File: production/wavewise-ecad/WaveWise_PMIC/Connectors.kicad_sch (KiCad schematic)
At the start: 30 parts, among them J1 5031590200, J10 5031590200, J11 5031590200, J13 Screw_Terminal_01x03, J2 Conn_01x06_Pin, J3 Conn_01x03_Pin, J5 5031590400, J6 5031590400, J8 5031590800, J9 5031590300

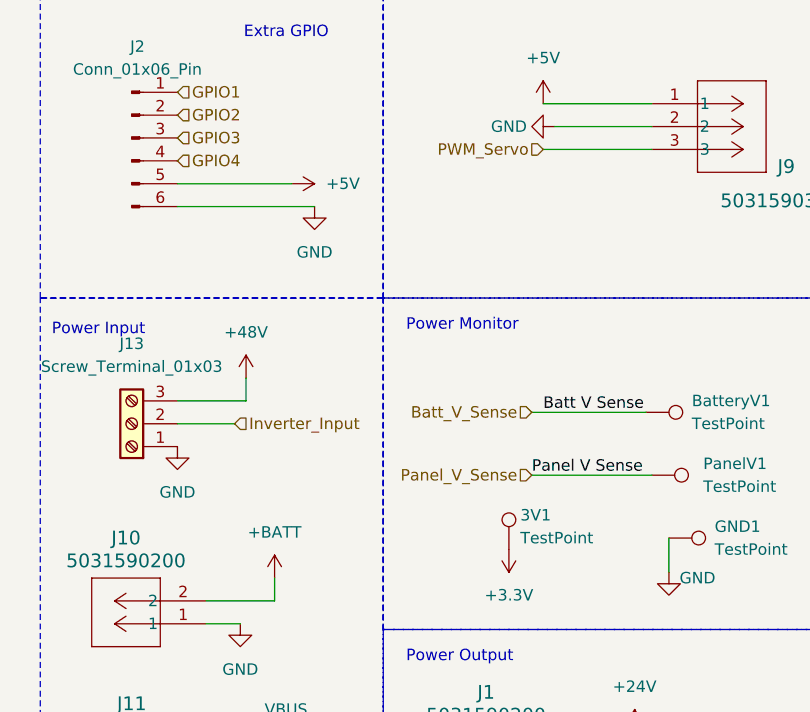
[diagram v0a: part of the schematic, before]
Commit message: add gerber files
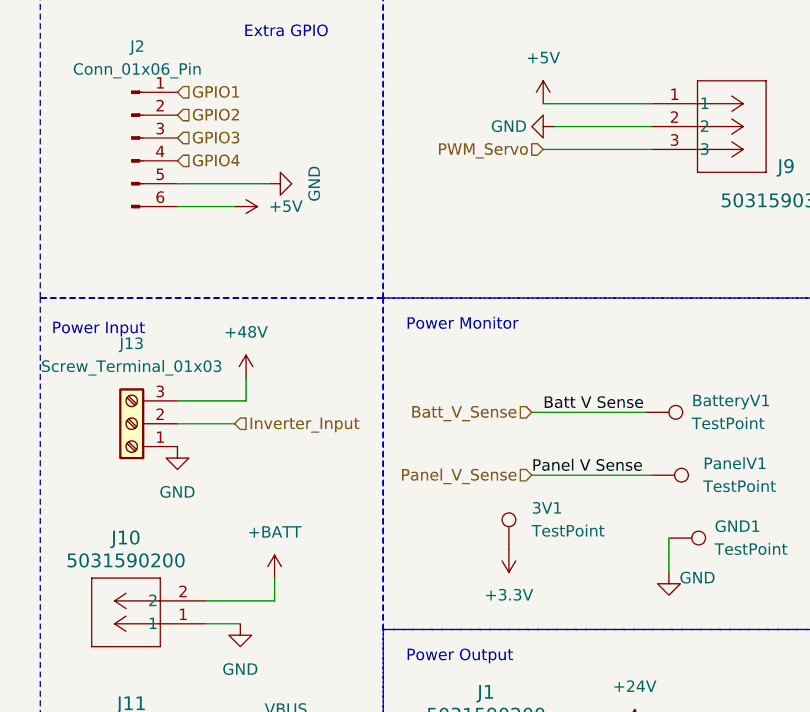
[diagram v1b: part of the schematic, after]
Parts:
- 3V1: footprint TestPoint:TestPoint_Pad_D1.5mm -> TestPoint:TestPoint_THTPad_D2.0mm_Drill1.0mm
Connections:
- net +5V: now also J2.6 (Pin_6); no longer J2.5 (Pin_5)
- net GND: now also J2.5 (Pin_5); no longer J2.6 (Pin_6)
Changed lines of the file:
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@@
   (junction (at 157.48 106.68) (diameter 0) (color 0 0 0 0)
+  )
+  (wire (pts (xy 27.94 39.37) (xy 34.29 39.37))
+    (stroke (width 0) (type default))
   )
   (polyline (pts (xy 105.41 123.19) (xy 105.41 126.746))
@@
     (stroke (width 0) (type default))
   )
+  (wire (pts (xy 27.94 36.83) (xy 38.1 36.83))
+    (stroke (width 0) (type default))
+  )
   (wire (pts (xy 78.74 138.43) (xy 78.74 139.7))
     (stroke (width 0) (type default))
@@
     (stroke (width 0) (type default))
   )
-  (wire (pts (xy 43.18 39.37) (xy 27.94 39.37))
-    (stroke (width 0) (type default))
-  )
   (wire (pts (xy 158.75 114.3) (xy 157.48 114.3))
     (stroke (width 0) (type default))
@@
   )
   (wire (pts (xy 120.904 84.328) (xy 128.016 84.328))
-    (stroke (width 0) (type default))
-  )
-  (wire (pts (xy 40.64 36.83) (xy 27.94 36.83))
     (stroke (width 0) (type default))
   )
@@
     )
   )
+  (symbol (lib_id "Connector:TestPoint") (at 64.77 77.47 0) (unit 1)
+    (in_bom yes) (on_board yes) (dnp no) (fields_autoplaced)
+    (property "Reference" "3V1" (at 67.31 72.898 0)
+      (effects (font (size 1.27 1.27)) (justify left))
+    )
+    (property "Value" "TestPoint" (at 67.31 75.438 0)
+      (effects (font (size 1.27 1.27)) (justify left))
+    )
+    (property "Footprint" "TestPoint:TestPoint_THTPad_D2.0mm_Drill1.0mm" (at 69.85 77.47 0)
+      (effects (font (size 1.27 1.27)) hide)
+    )
+    (property "Datasheet" "~" (at 69.85 77.47 0)
+      (effects (font (size 1.27 1.27)) hide)
+    )
+    (pin "1")
+    (instances
+      (project "WaveWise_PMIC"
+        (path "/8343c01b-8940-4cb8-a17d-91fd7fb1cccd/7fd42481-dc5a-4ae0-adec-c5e7a3228be9"
+          (reference "3V1") (unit 1)
+        )
+      )
+    )
+  )
   (symbol (lib_id "Connector:TestPoint") (at 80.01 62.23 270) (unit 1)
     (in_bom yes) (on_board yes) (dnp no) (fields_autoplaced)
@@
     )
   )
-  (symbol (lib_id "power:+5V") (at 40.64 36.83 270) (unit 1)
-    (in_bom yes) (on_board yes) (dnp no) (fields_autoplaced)
-    (property "Reference" "#PWR01" (at 36.83 36.83 0)
-      (effects (font (size 1.27 1.27)) hide)
-    )
-    (property "Value" "+5V" (at 44.45 36.83 90)
+  (symbol (lib_id "power:+5V") (at 34.29 39.37 270) (unit 1)
+    (in_bom yes) (on_board yes) (dnp no) (fields_autoplaced)
+    (property "Reference" "#PWR01" (at 30.48 39.37 0)
+      (effects (font (size 1.27 1.27)) hide)
+    )
+    (property "Value" "+5V" (at 38.1 39.37 90)
       (effects (font (size 1.27 1.27)) (justify left))
     )
-    (property "Footprint" "" (at 40.64 36.83 0)
-      (effects (font (size 1.27 1.27)) hide)
-    )
-    (property "Datasheet" "" (at 40.64 36.83 0)
+    (property "Footprint" "" (at 34.29 39.37 0)
+      (effects (font (size 1.27 1.27)) hide)
+    )
+    (property "Datasheet" "" (at 34.29 39.37 0)
       (effects (font (size 1.27 1.27)) hide)
     )
@@
     )
   )
-  (symbol (lib_id "power:GND") (at 43.18 39.37 0) (unit 1)
+  (symbol (lib_id "power:GND") (at 38.1 36.83 90) (unit 1)
     (in_bom yes) (on_board yes) (dnp no)
-    (property "Reference" "#PWR05" (at 43.18 45.72 0)
-      (effects (font (size 1.27 1.27)) hide)
-    )
-    (property "Value" "GND" (at 43.18 44.45 0)
-      (effects (font (size 1.27 1.27)))
-    )
-    (property "Footprint" "" (at 43.18 39.37 0)
-      (effects (font (size 1.27 1.27)) hide)
-    )
-    (property "Datasheet" "" (at 43.18 39.37 0)
+    (property "Reference" "#PWR05" (at 44.45 36.83 0)
+      (effects (font (size 1.27 1.27)) hide)
+    )
+    (property "Value" "GND" (at 43.18 36.83 0)
+      (effects (font (size 1.27 1.27)))
+    )
+    (property "Footprint" "" (at 38.1 36.83 0)
+      (effects (font (size 1.27 1.27)) hide)
+    )
+    (property "Datasheet" "" (at 38.1 36.83 0)
       (effects (font (size 1.27 1.27)) hide)
     )
@@
         )
       )
-    )
-  )
-  (symbol (lib_id "Connector:TestPoint") (at 64.77 77.47 0) (unit 1)
-    (in_bom yes) (on_board yes) (dnp no)
-    (property "Reference" "3V1" (at 66.04 73.66 0)
-      (effects (font (size 1.27 1.27)) (justify left))
-    )
-    (property "Value" "TestPoint" (at 66.04 76.2 0)
-      (effects (font (size 1.27 1.27)) (justify left))
-    )
-    (property "Footprint" "TestPoint:TestPoint_Pad_D1.5mm" (at 69.85 77.47 0)
-      (effects (font (size 1.27 1.27)) hide)
-    )
-    (property "Datasheet" "~" (at 69.85 77.47 0)
-      (effects (font (size 1.27 1.27)) hide)
-    )
-    (pin "1")
-    (instances
-      (project "WaveWise_PMIC"
-        (path "/8343c01b-8940-4cb8-a17d-91fd7fb1cccd/7fd42481-dc5a-4ae0-adec-c5e7a3228be9"
-          (reference "3V1") (unit 1)
-        )
-      )
